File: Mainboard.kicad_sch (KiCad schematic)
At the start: 25 parts, among them J1 Conn_02x04_Odd_Even, J10 Barrel_Jack_Switch, J2 Conn_02x04_Odd_Even, J3 Conn_02x04_Odd_Even, J4 Conn_02x04_Odd_Even, J5 Conn_01x04_Socket, J6 Conn_01x04_Socket, J7 Conn_01x04_Socket, J8 Conn_01x04_Socket, SW1 SW_SPDT, U1 ESP32-DEVKIT-V1, U2 MP2303ADN, U3 AMS1117-3.3

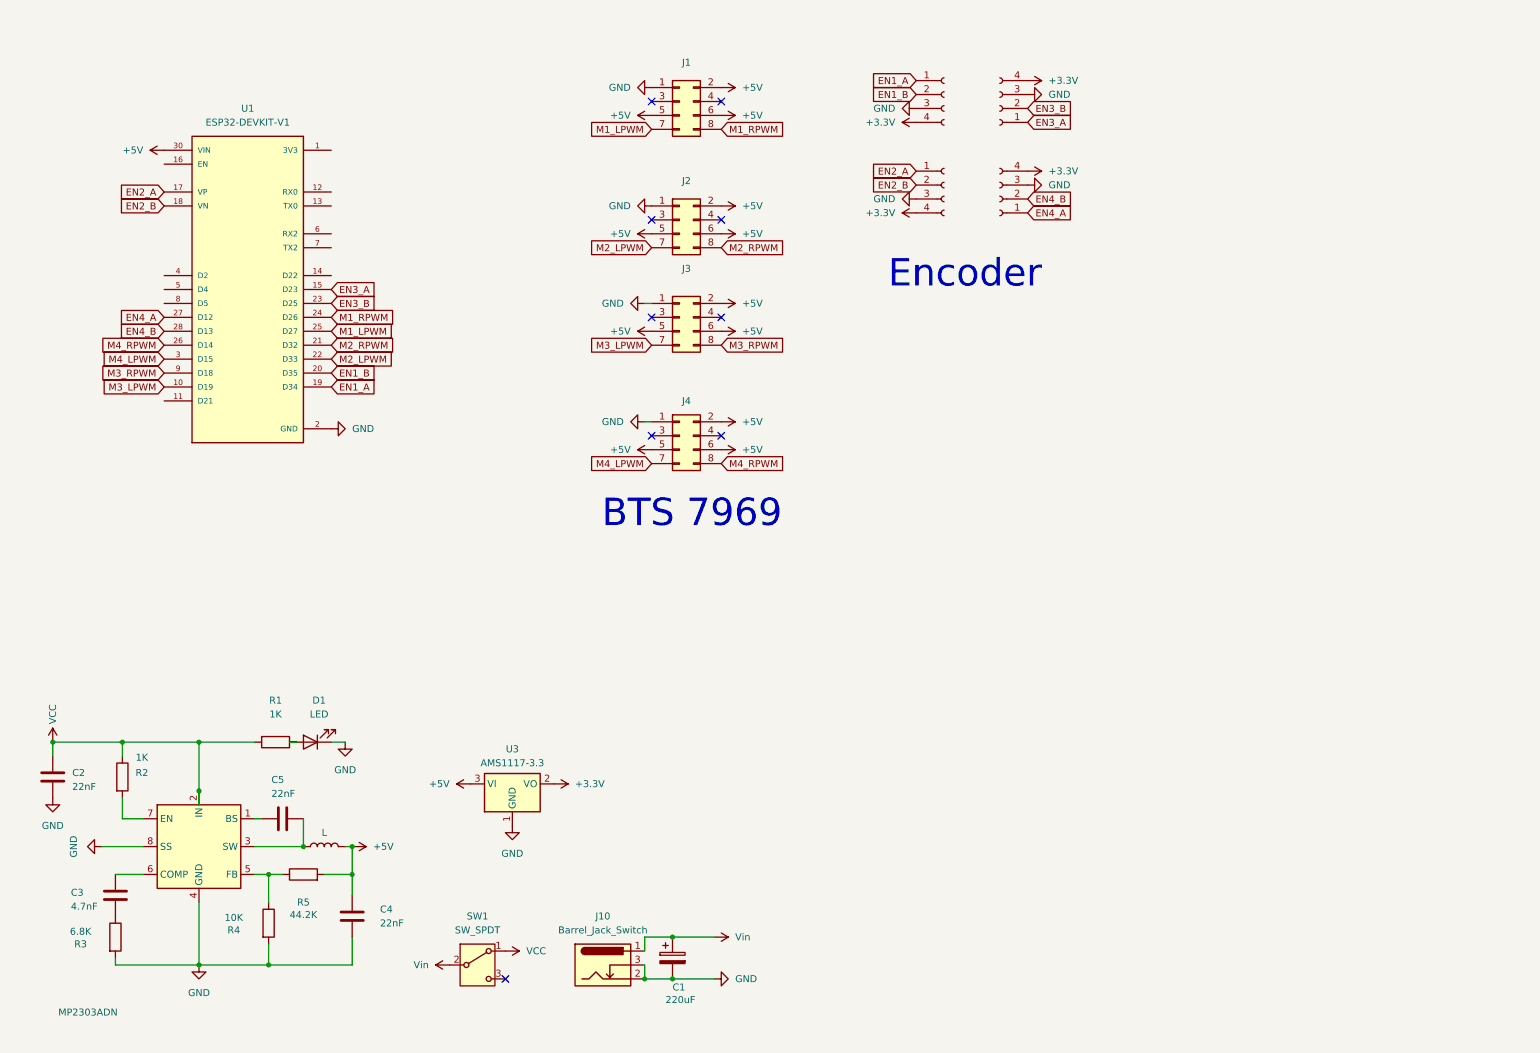
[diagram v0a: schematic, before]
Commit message: done
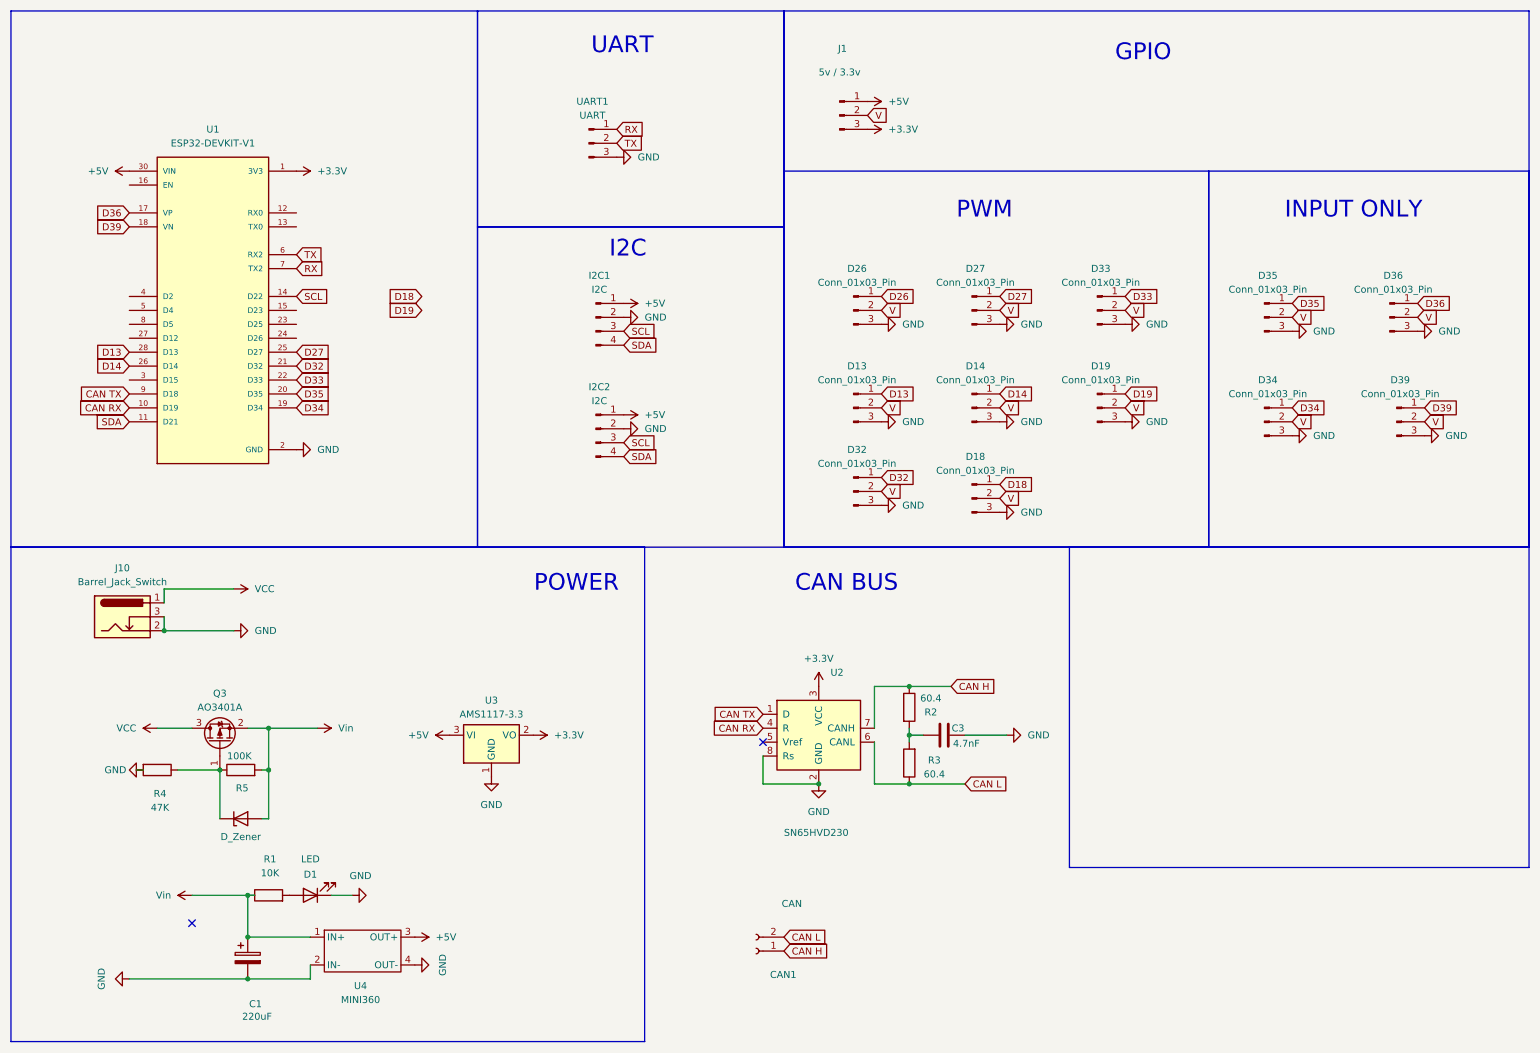
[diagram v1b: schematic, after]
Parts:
- removed C2, C4, C5: 22nF, symbol Device:C
- removed J1, J2, J3, J4: Conn_02x04_Odd_Even, Connector_IDC:IDC-Header_2x04_P2.54mm_Vertical, symbol Connector_Generic:Conn_02x04_Odd_Even
- removed J5, J6, J7, J8: Conn_01x04_Socket, Connector_JST:JST_XH_B4B-XH-A_1x04_P2.50mm_Vertical, symbol Connector:Conn_01x04_Socket
- removed L1: L, symbol Device:L
- removed SW1: SW_SPDT, symbol Switch:SW_SPDT
- removed U2: MP2303ADN, Package_SO:SOIC-8-1EP_3.9x4.9mm_P1.27mm_EP2.62x3.51mm, symbol Regulator_Switching:MP2303ADN
- added CAN1: CAN, Connector_PinHeader_2.54mm:PinHeader_1x02_P2.54mm_Vertical, symbol Connector:Conn_01x02_Socket
- added D13, D14, D18, D19, D26, D27, D32, D33, D34, D35, D36, D39: Conn_01x03_Pin, Connector_PinHeader_2.54mm:PinHeader_1x03_P2.54mm_Vertical, symbol Connector:Conn_01x03_Pin
- added D2: D_Zener, Diode_THT:D_DO-41_SOD81_P10.16mm_Horizontal, symbol Device:D_Zener
- added I2C1, I2C2: I2C, Connector_PinHeader_2.54mm:PinHeader_1x04_P2.54mm_Vertical, symbol Connector:Conn_01x04_Pin
- added J1: 5v / 3.3v, Connector_PinHeader_2.54mm:PinHeader_1x03_P2.54mm_Vertical, symbol Connector:Conn_01x03_Pin
- added Q3: AO3401A, Package_TO_SOT_SMD:SOT-23, symbol Transistor_FET:AO3401A
- added U2: SN65HVD230, Package_SO:SOIC-8_3.9x4.9mm_P1.27mm, symbol Interface_CAN_LIN:SN65HVD230
- added U4: MINI360, MINI360:Mini360, symbol New_Library:Mini360
- added UART1: UART, Connector_PinHeader_2.54mm:PinHeader_1x03_P2.54mm_Vertical, symbol Connector:Conn_01x03_Pin
- C1: footprint (none) -> Capacitor_SMD:CP_Elec_8x10.5
- C3: footprint (none) -> Capacitor_SMD:C_0805_2012Metric_Pad1.18x1.45mm_HandSolder
- D1: footprint (none) -> LED_SMD:LED_1206_3216Metric_Pad1.42x1.75mm_HandSolder
- J10: footprint (none) -> Connector_BarrelJack:BarrelJack_Horizontal
- R1: value 1K -> 10K; footprint (none) -> Resistor_SMD:R_0805_2012Metric_Pad1.20x1.40mm_HandSolder
- R2: value 1K -> 60.4; footprint (none) -> Resistor_SMD:R_0805_2012Metric_Pad1.20x1.40mm_HandSolder
- R3: value 6.8K -> 60.4; footprint (none) -> Resistor_SMD:R_0805_2012Metric_Pad1.20x1.40mm_HandSolder
- R4: value 10K -> 47K; footprint (none) -> Resistor_SMD:R_0805_2012Metric_Pad1.20x1.40mm_HandSolder
- R5: value 44.2K -> 100K; footprint (none) -> Resistor_SMD:R_0805_2012Metric_Pad1.20x1.40mm_HandSolder
- U1: footprint ESP32-DEVKIT-V1:MODULE_ESP32_DEVKIT_V1 -> ESP32:MODULE_ESP32_DEVKIT_V1
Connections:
- net +3.3V: now also U1.1 (3V3), J1.3 (Pin_3), U2.3 (VCC)
- net +5V: now also I2C1.1 (Pin_1), I2C2.1 (Pin_1), J1.1 (Pin_1), U4.3 (OUT+); no longer R5.2
- net GND: now also C3.2, D13.3 (Pin_3), D14.3 (Pin_3), D18.3 (Pin_3), D19.3 (Pin_3), D26.3 (Pin_3), D27.3 (Pin_3), D32.3 (Pin_3), D33.3 (Pin_3), D34.3 (Pin_3), D35.3 (Pin_3), D36.3 (Pin_3), D39.3 (Pin_3), I2C1.2 (Pin_2), I2C2.2 (Pin_2), U2.2 (GND), U2.8 (Rs), U4.2 (IN-), U4.4 (OUT-), UART1.3 (Pin_3); no longer R3.2
- net VCC: now also J10.1, Q3.3 (D); no longer R1.2, R2.1
- net Vin: now also R1.1, R5.2, D2.2 (A), Q3.2 (S), U4.1 (IN+); no longer J10.1
- net at R4.1, R5.1: now also D2.1 (K), Q3.1 (G)
- net at D1.2 (A): now also R1.2; no longer R1.1
- net at C3.1: now also R2.2, R3.2
- net SDA: now reaches U1.11 (D21)
- net SDA: now also I2C1.4 (Pin_4), I2C2.4 (Pin_4)
- net SCL: now reaches U1.14 (D22)
- net SCL: now also I2C1.3 (Pin_3), I2C2.3 (Pin_3)
- net TX: now reaches U1.6 (RX2)
- net TX: now also UART1.2 (Pin_2)
- net RX: now reaches U1.7 (TX2)
- net RX: now also UART1.1 (Pin_1)
- net CAN L: now reaches R3.1
- net CAN L: now also CAN1.2 (Pin_2), U2.6 (CANL); no longer C3.2
- net EN1_A renamed D34
- net D34: now also D34.1 (Pin_1)
- net EN1_B renamed D35
- net D35: now also D35.1 (Pin_1)
- net EN2_A renamed D36
- net D36: now also D36.1 (Pin_1)
- net EN2_B renamed D39
- net D39: now also D39.1 (Pin_1)
- net EN3_A: no longer names the net of U1.15 (D23)
- net EN3_B: no longer names the net of U1.23 (D25)
- net EN4_A: no longer names the net of U1.27 (D12)
- net EN4_B renamed D13
- net D13: now also D13.1 (Pin_1)
- net M1_LPWM renamed D27
- net D27: now also D27.1 (Pin_1)
- net M1_RPWM: no longer names the net of U1.24 (D26)
- net M2_LPWM renamed D33
- net D33: now also D33.1 (Pin_1)
- net M2_RPWM renamed D32
- net D32: now also D32.1 (Pin_1)
- net M3_LPWM renamed CAN RX
- net CAN RX: now also U2.4 (R)
- net M3_RPWM renamed CAN TX
- net CAN TX: now also U2.1 (D)
- net M4_LPWM: no longer names the net of U1.3 (D15)
- net M4_RPWM renamed D14
- net D14: now also D14.1 (Pin_1)
- new net CAN H: CAN1.1 (Pin_1), R2.1, U2.7 (CANH)
- new net D18: D18.1 (Pin_1)
- new net D19: D19.1 (Pin_1)
- new net D26: D26.1 (Pin_1)
- new net V: D13.2 (Pin_2), D14.2 (Pin_2), D18.2 (Pin_2), D19.2 (Pin_2), D26.2 (Pin_2), D27.2 (Pin_2), D32.2 (Pin_2), D33.2 (Pin_2), D34.2 (Pin_2), D35.2 (Pin_2), D36.2 (Pin_2), D39.2 (Pin_2), J1.2 (Pin_2)
- no-connect marks 9 -> 2
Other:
- note added: "CAN BUS"
- note added: "GPIO"
- note added: "I2C"
- note added: "INPUT ONLY"
- note added: "POWER"
- note added: "PWM"
- note added: "UART"
- note removed: "BTS 7969"
- note removed: "Encoder"
- moved on the sheet: J10, U1, U3
